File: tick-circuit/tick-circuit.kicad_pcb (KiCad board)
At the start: 2 copper layers, 45.7 x 33 mm, 14 parts, among them J1 Power, J2 50/60Hz, U1 74HCT4060, U2 74HCT73, X1 3.93216 MHz

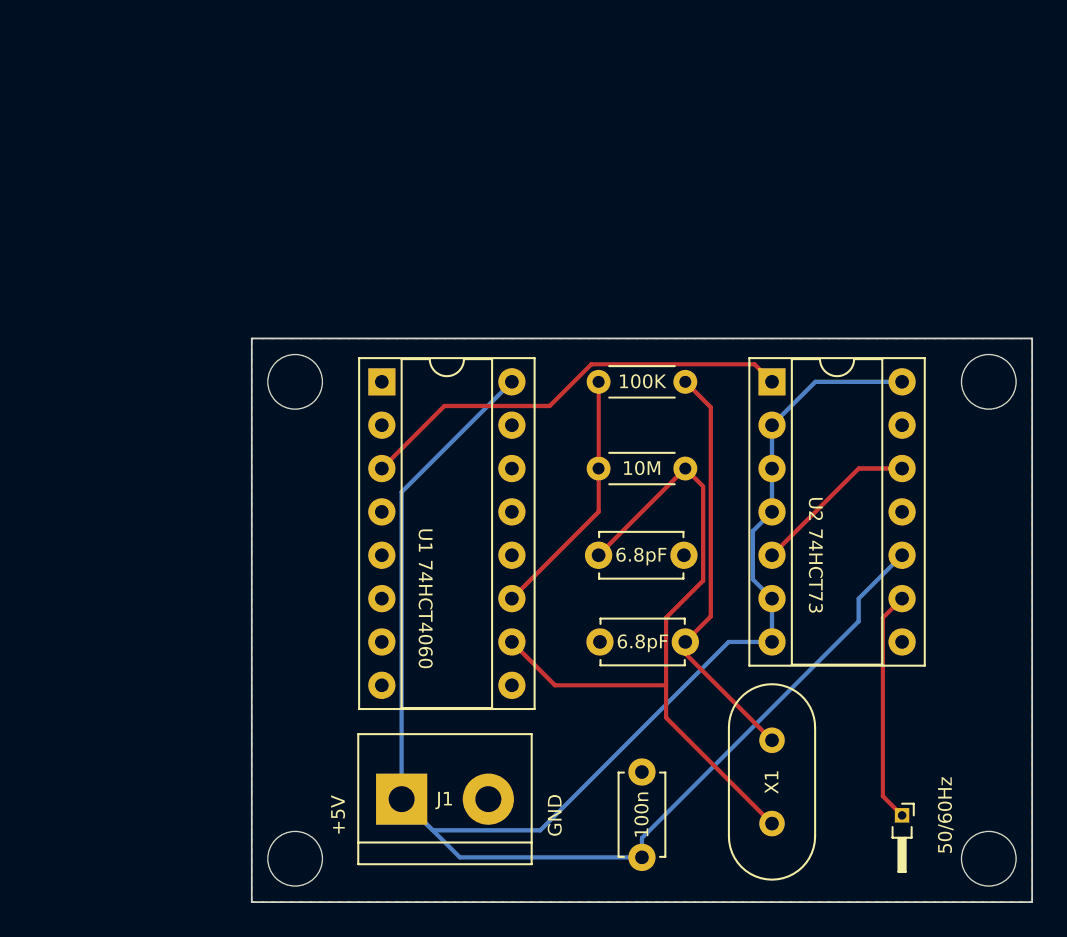
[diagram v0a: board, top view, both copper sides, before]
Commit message: I like to move it move it
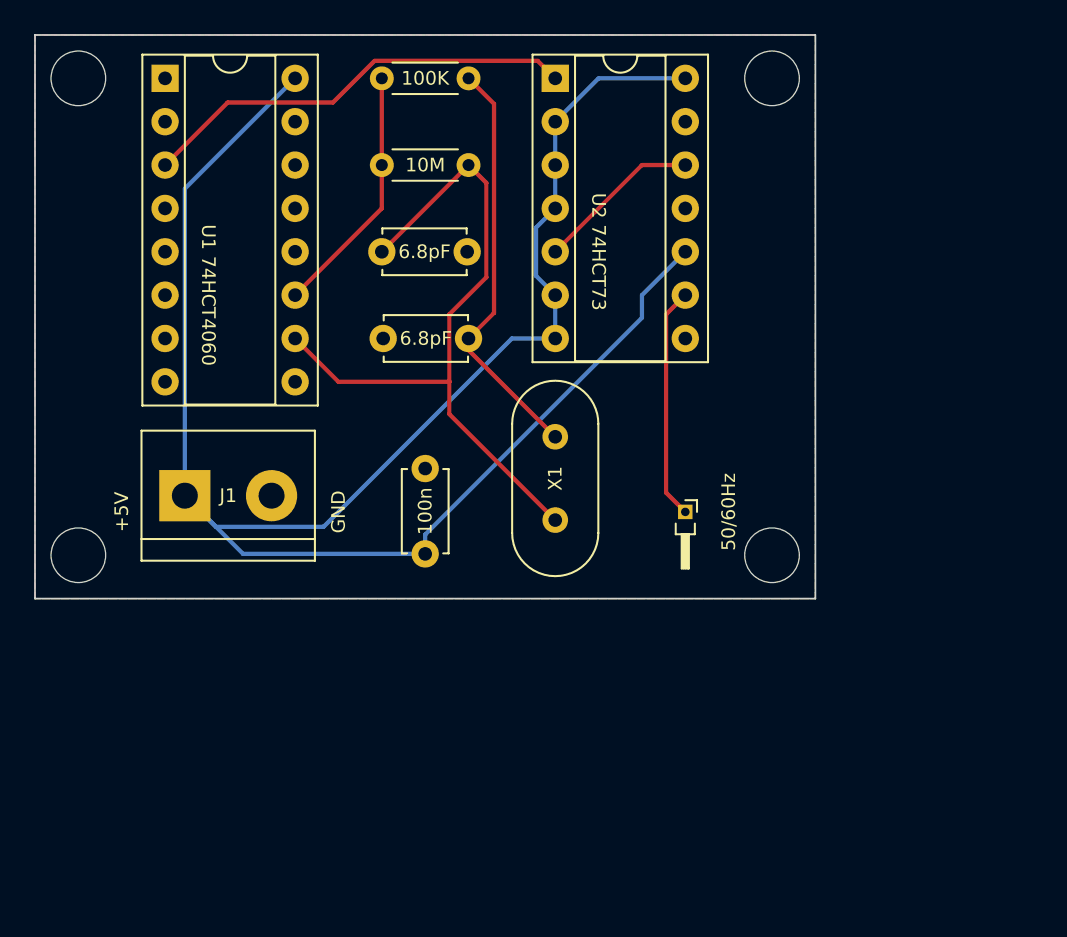
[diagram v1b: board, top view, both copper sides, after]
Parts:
- moved J2 21.8 mm to (50.8, 40.6)
- moved U1 21.8 mm to (20.3, 15.2)
- moved U2 21.8 mm to (43.2, 15.2)
- moved X1 21.8 mm to (43.2, 41.1)
- moved J1 21.8 mm to (21.5, 39.7)
- moved REF** 21.8 mm to (15.2, 43.2)
- moved REF** 21.8 mm to (15.2, 15.2)
- moved C1 21.8 mm to (33.0, 25.4)
- moved C2 21.8 mm to (38.1, 30.5)
- moved C3 21.8 mm to (35.6, 43.1)
- moved R1 21.8 mm to (38.1, 20.3)
- moved R2 21.8 mm to (33.0, 15.2)
- moved REF** 21.8 mm to (55.9, 43.2)
- moved REF** 21.8 mm to (55.9, 15.2)
